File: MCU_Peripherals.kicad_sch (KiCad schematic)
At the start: 45 parts, among them J1 USB_C_Receptacle_USB2.0_16P, J2 Conn_01x02_Socket, J3 Conn_01x04_Pin, U2 SN65HVD230DR, U3 USBLC6-2SC6, U4 M24C64-RMN6TP, Y1 Crystal_16MHz

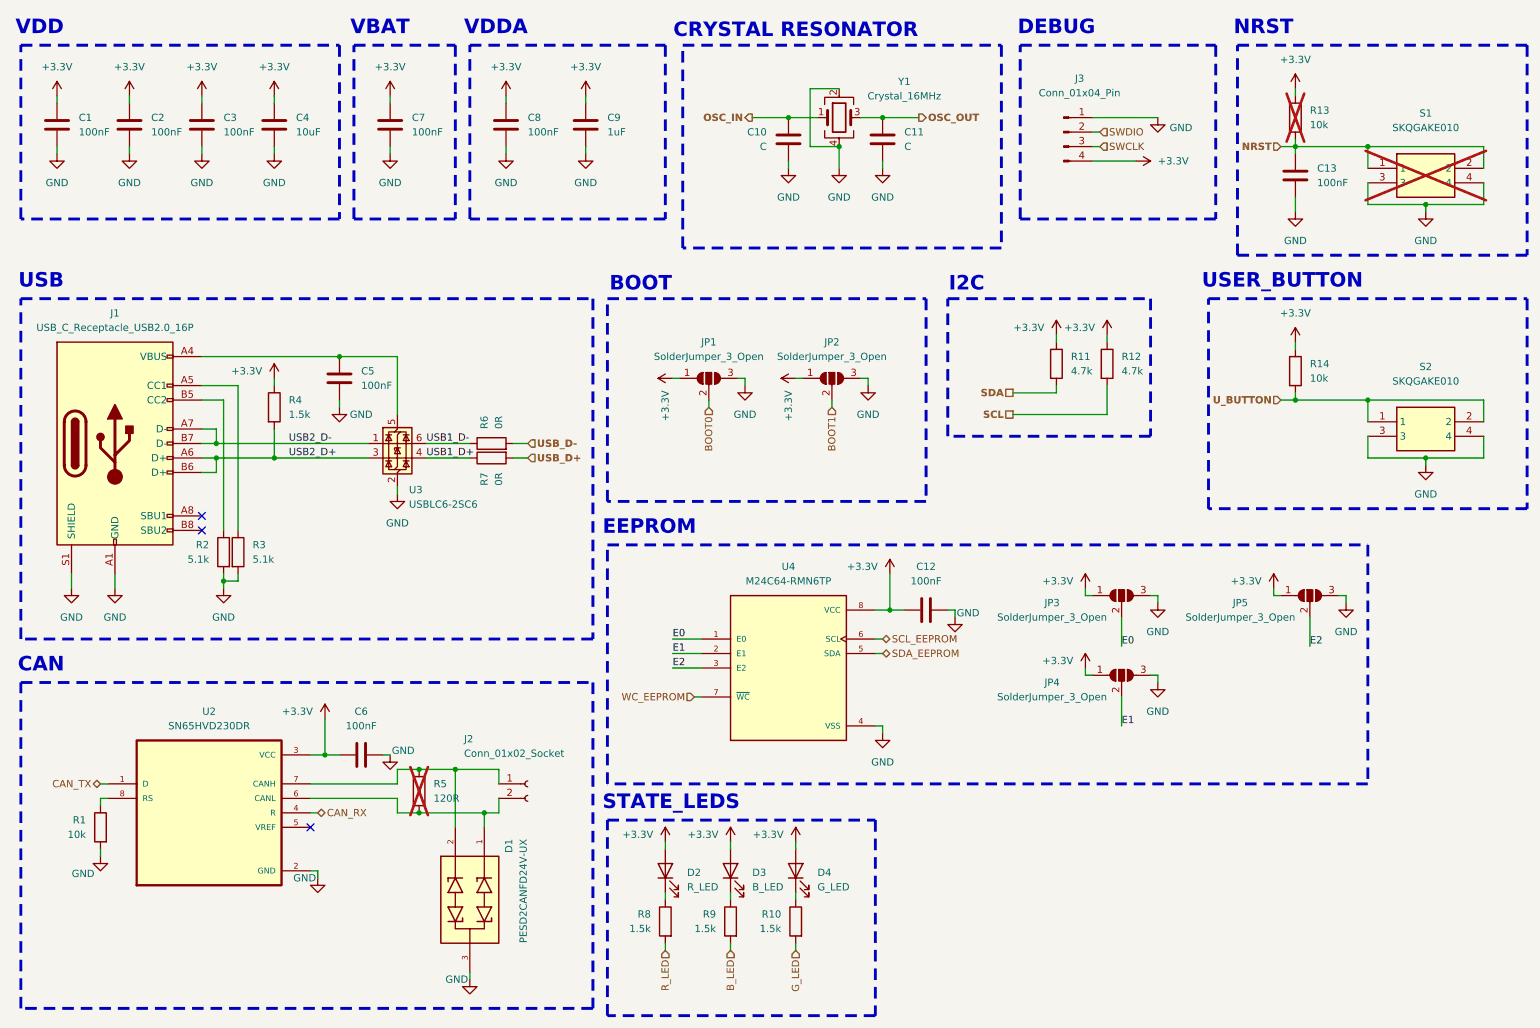
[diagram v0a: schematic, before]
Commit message: Layout Update
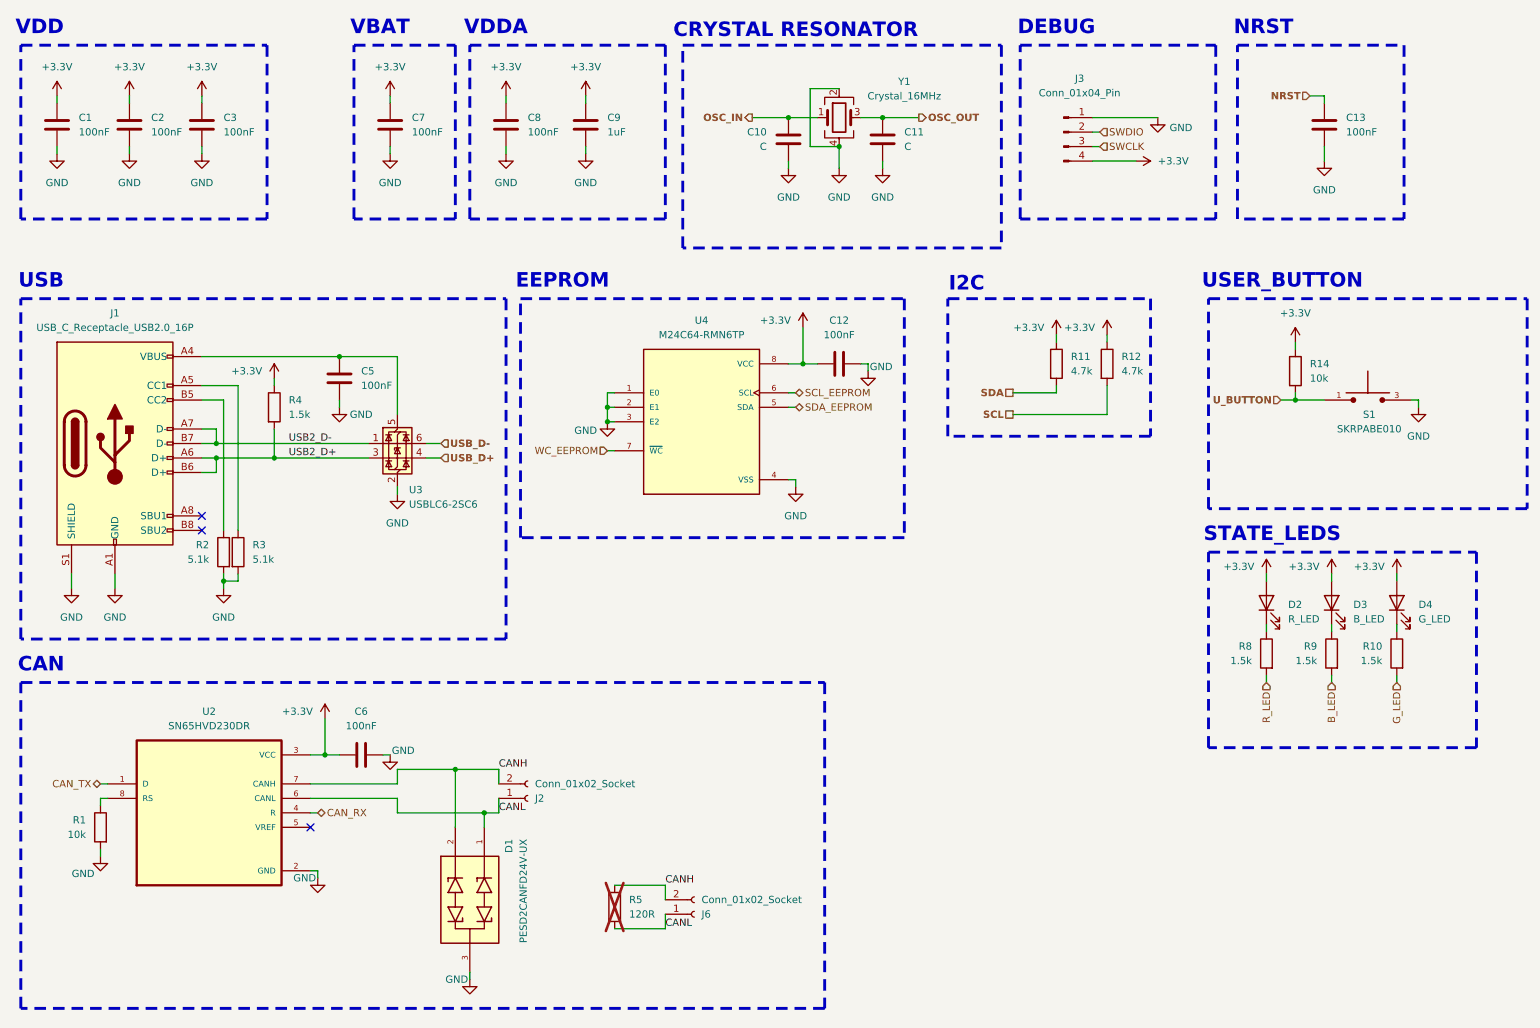
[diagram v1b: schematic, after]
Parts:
- removed C4: 10uF, Capacitor_SMD:C_0402_1005Metric_Pad0.74x0.62mm_HandSolder, symbol Device:C
- removed JP1, JP2, JP3, JP4, JP5: SolderJumper_3_Open, Jumper:SolderJumper-3_P1.3mm_Open_RoundedPad1.0x1.5mm_NumberLabels, symbol Jumper:SolderJumper_3_Open
- removed R13: 10k, Resistor_SMD:R_0402_1005Metric_Pad0.72x0.64mm_HandSolder, symbol Device:R
- removed R6, R7: 0R, Resistor_SMD:R_0402_1005Metric_Pad0.72x0.64mm_HandSolder, symbol Device:R
- removed S1, S2: SKQGAKE010, KSZ_KiCad_Footprint_Library:SKQGAKE010, symbol KSZ_KiCad_Symbol_Library:SKQGAKE010
- added J6: Conn_01x02_Socket, Connector_JST:JST_PH_S2B-PH-K_1x02_P2.00mm_Horizontal, symbol Connector:Conn_01x02_Socket
- added S1: SKRPABE010, KSZ_KiCad_Footprint_Library:SW_SKRPABE010, symbol KSZ_KiCad_Symbol_Library:SKRPABE010
- J2: footprint TerminalBlock:TerminalBlock_MaiXu_MX126-5.0-02P_1x02_P5.00mm -> Connector_JST:JST_PH_S2B-PH-K_1x02_P2.00mm_Horizontal
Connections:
- net E0 is gone; now on net GND: U4.1 (E0)
- net E1 is gone; now on net GND: U4.2 (E1)
- net E2 is gone; now on net GND: U4.3 (E2)
- net USB1_D+ is gone; now on net USB_D+: U3.4 (I/O2)
- net USB1_D- is gone; now on net USB_D-: U3.6 (I/O1)
- net GND: now also S1.3, S1.4
- net U_BUTTON: now also S1.1, S1.2
- net CANL: now reaches D1.1, R5.2, U2.6 (CANL)
- net CANL: now also J2.1 (Pin_1), J6.1 (Pin_1); no longer J2.2 (Pin_2)
- net CANH: now reaches D1.2, R5.1, U2.7 (CANH)
- net CANH: now also J2.2 (Pin_2), J6.2 (Pin_2); no longer J2.1 (Pin_1)
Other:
- note removed: "BOOT"
- moved on the sheet: C12, C13, D2, D3, D4, R10, R5, R8, R9, U4
